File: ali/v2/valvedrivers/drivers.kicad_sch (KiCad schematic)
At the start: 24 parts, among them J10 Conn_01x02, J11 Conn_01x02, J12 Conn_01x02, J13 Conn_01x02, U6 IPS4140HQ, U7 PS2841-4B, U8 PS2841-4B

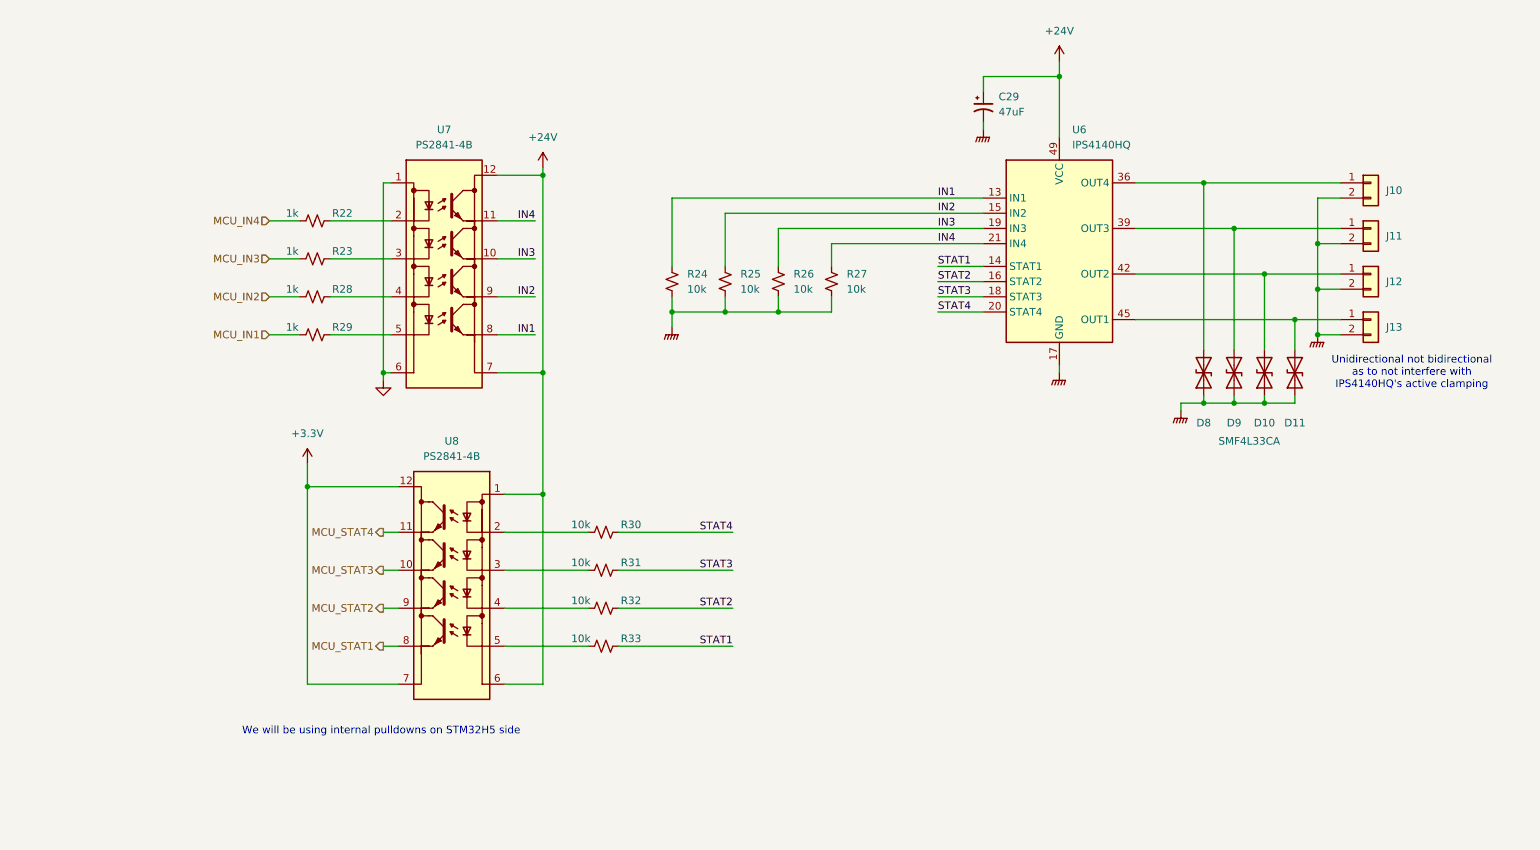
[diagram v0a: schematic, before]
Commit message: Commentary
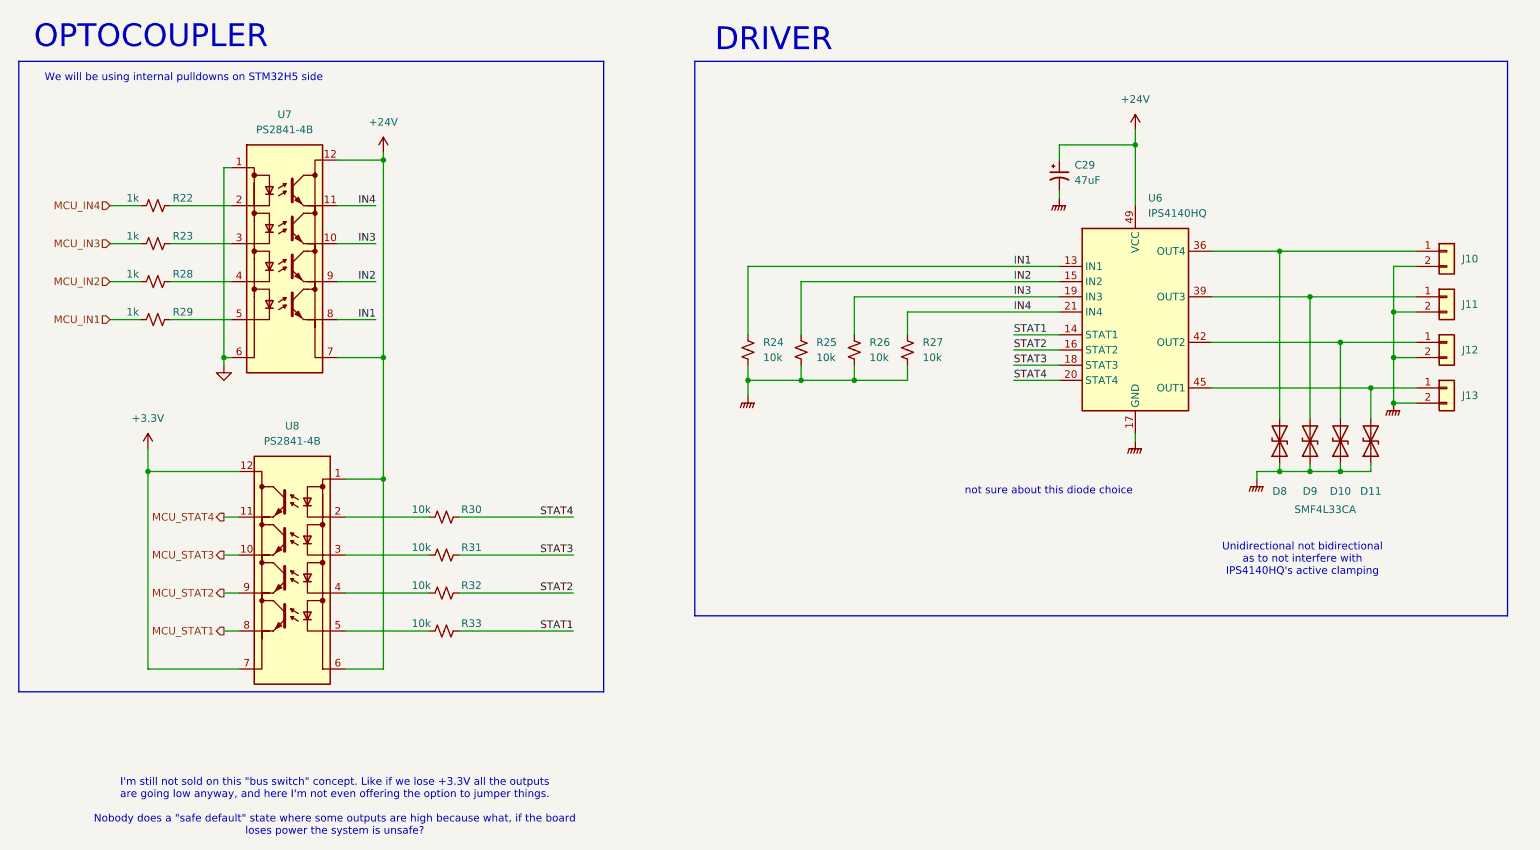
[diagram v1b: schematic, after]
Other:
- note added: "DRIVER"
- note added: "I'm still not sold on this "bus switch" concept. Like if we lose +3.3V all the outputs are going low anyway, and here I'm not even offering the option to jumper things. Nobody does a "safe default" state where some outputs are high because what, if the board loses power the system is unsafe?"
- note added: "OPTOCOUPLER"
- note added: "not sure about this diode choice"
- moved on the sheet: C29, D10, D11, D8, D9, J10, J11, J12, J13, R22, R23, R24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
